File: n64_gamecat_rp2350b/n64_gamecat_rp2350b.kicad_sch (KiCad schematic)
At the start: 3 parts, among them U4 RP235x-B

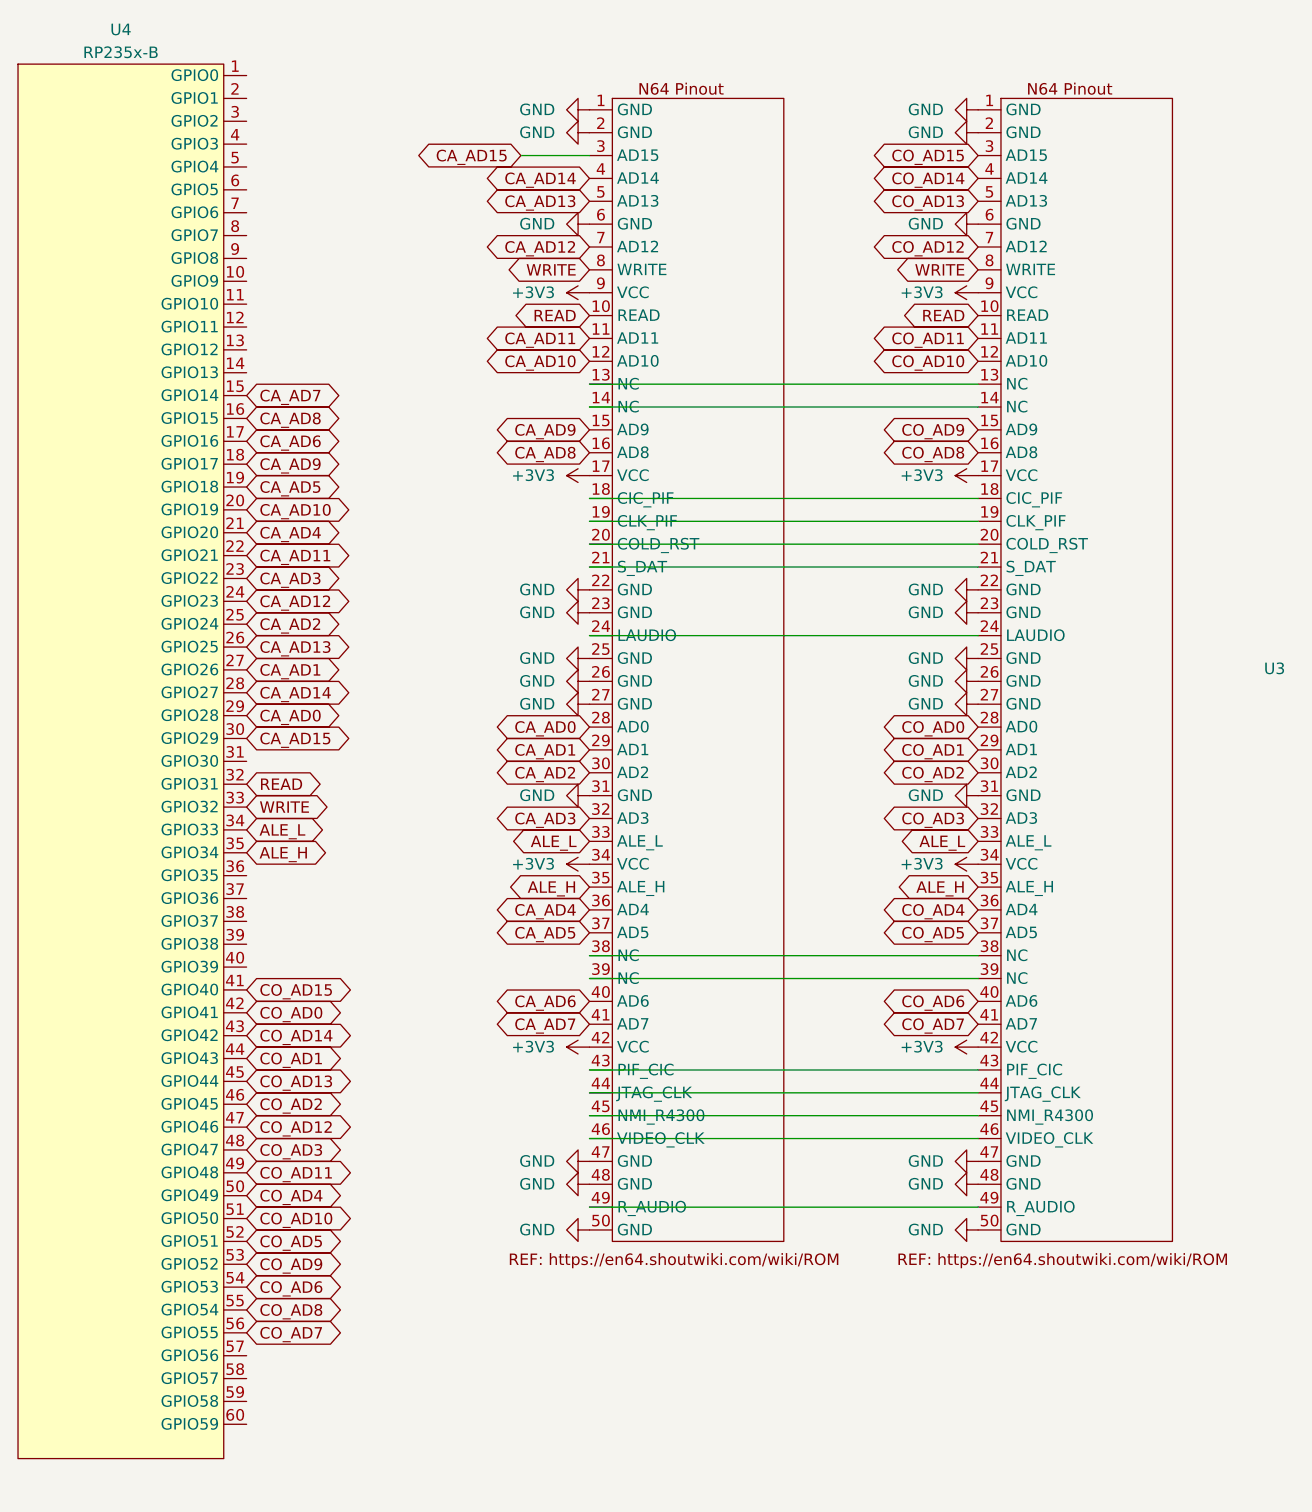
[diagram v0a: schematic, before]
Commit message: V0.6 PCB
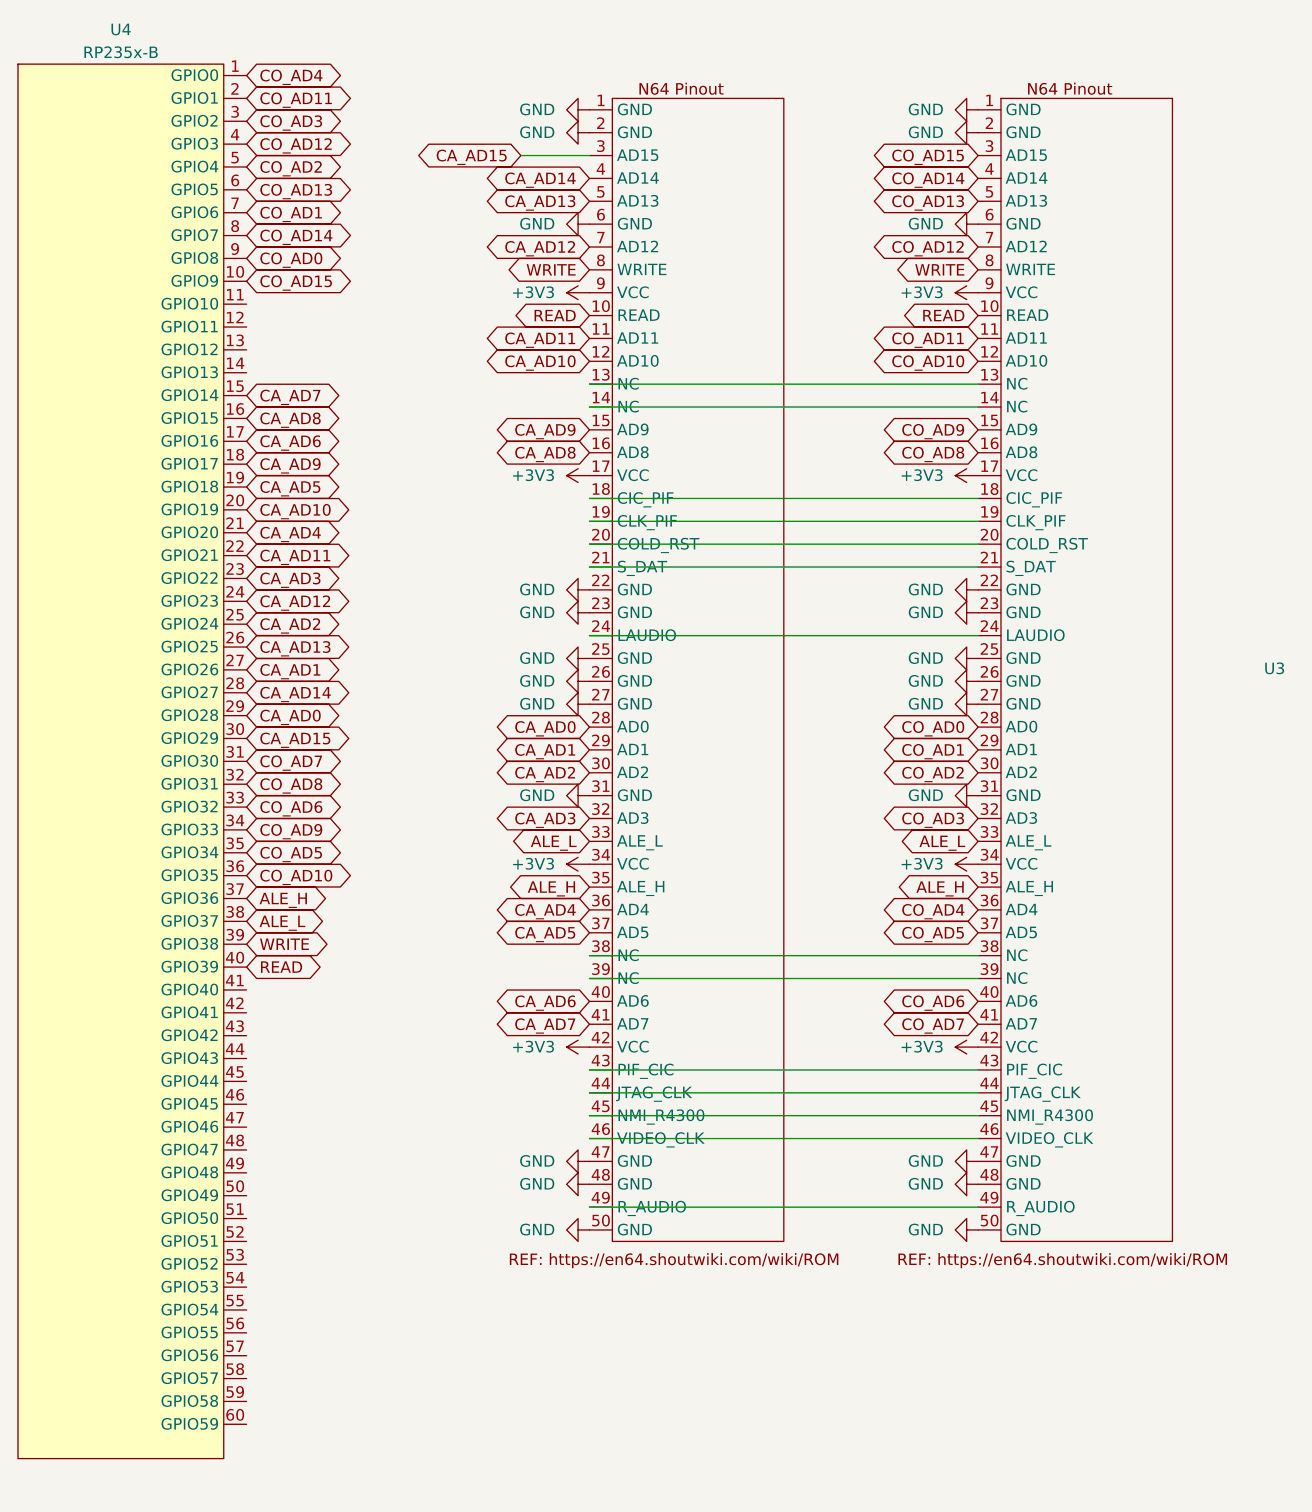
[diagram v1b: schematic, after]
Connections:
- net ALE_H: now also U4.37 (GPIO36); no longer U4.35 (GPIO34)
- net ALE_L: now also U4.38 (GPIO37); no longer U4.34 (GPIO33)
- net CO_AD0: now also U4.9 (GPIO8); no longer U4.42 (GPIO41)
- net CO_AD1: now also U4.7 (GPIO6); no longer U4.44 (GPIO43)
- net CO_AD10: now also U4.36 (GPIO35); no longer U4.51 (GPIO50)
- net CO_AD11: now also U4.2 (GPIO1); no longer U4.49 (GPIO48)
- net CO_AD12: now also U4.4 (GPIO3); no longer U4.47 (GPIO46)
- net CO_AD13: now also U4.6 (GPIO5); no longer U4.45 (GPIO44)
- net CO_AD14: now also U4.8 (GPIO7); no longer U4.43 (GPIO42)
- net CO_AD15: now also U4.10 (GPIO9); no longer U4.41 (GPIO40)
- net CO_AD2: now also U4.5 (GPIO4); no longer U4.46 (GPIO45)
- net CO_AD3: now also U4.3 (GPIO2); no longer U4.48 (GPIO47)
- net CO_AD4: now also U4.1 (GPIO0); no longer U4.50 (GPIO49)
- net CO_AD5: now also U4.35 (GPIO34); no longer U4.52 (GPIO51)
- net CO_AD6: now also U4.33 (GPIO32); no longer U4.54 (GPIO53)
- net CO_AD7: now also U4.31 (GPIO30); no longer U4.56 (GPIO55)
- net CO_AD8: now also U4.32 (GPIO31); no longer U4.55 (GPIO54)
- net CO_AD9: now also U4.34 (GPIO33); no longer U4.53 (GPIO52)
- net READ: now also U4.40 (GPIO39); no longer U4.32 (GPIO31)
- net WRITE: now also U4.39 (GPIO38); no longer U4.33 (GPIO32)

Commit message: v0.7 PCB; prep for 2350
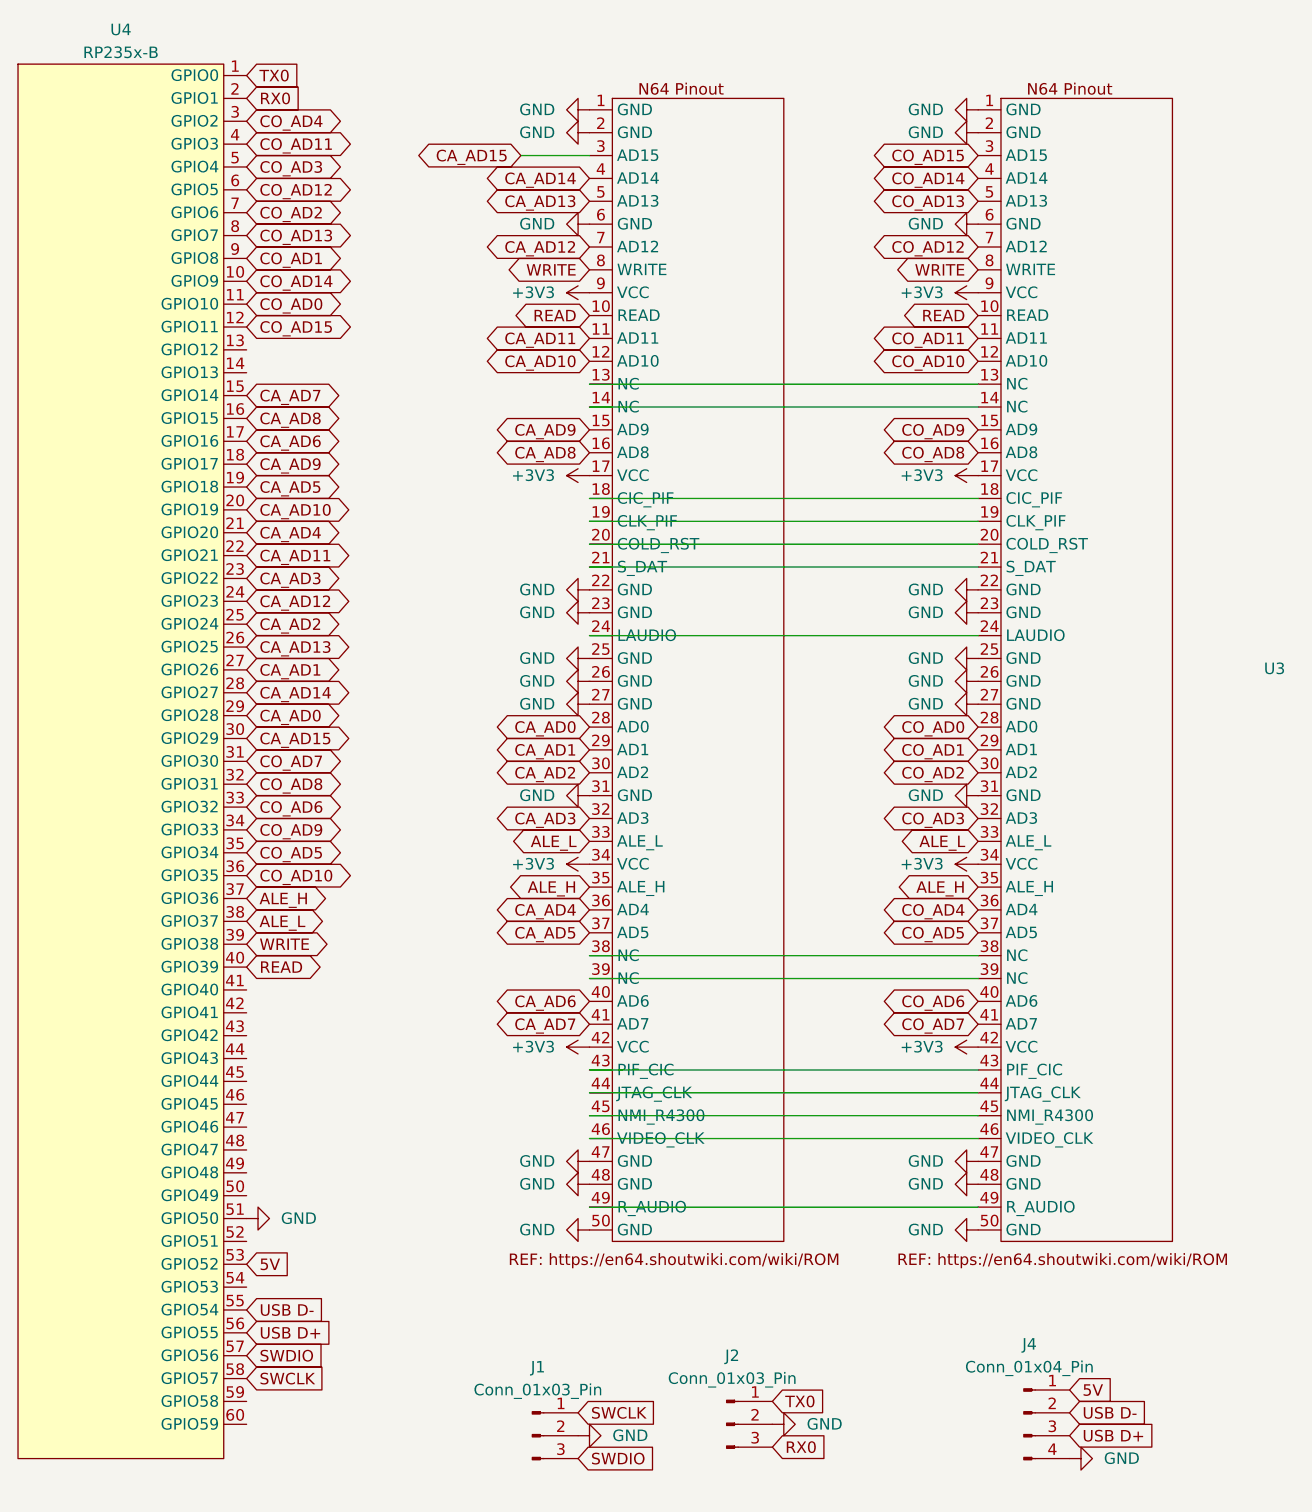
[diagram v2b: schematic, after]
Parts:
- added J1, J2: Conn_01x03_Pin, Connector_PinHeader_2.54mm:PinHeader_1x03_P2.54mm_Vertical, symbol Connector:Conn_01x03_Pin
- added J4: Conn_01x04_Pin, Connector_PinSocket_2.54mm:PinSocket_1x04_P2.54mm_Vertical, symbol Connector:Conn_01x04_Pin
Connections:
- net CO_AD0: now also U4.11 (GPIO10); no longer U4.9 (GPIO8)
- net CO_AD1: now also U4.9 (GPIO8); no longer U4.7 (GPIO6)
- net CO_AD11: now also U4.4 (GPIO3); no longer U4.2 (GPIO1)
- net CO_AD12: now also U4.6 (GPIO5); no longer U4.4 (GPIO3)
- net CO_AD13: now also U4.8 (GPIO7); no longer U4.6 (GPIO5)
- net CO_AD14: now also U4.10 (GPIO9); no longer U4.8 (GPIO7)
- net CO_AD15: now also U4.12 (GPIO11); no longer U4.10 (GPIO9)
- net CO_AD2: now also U4.7 (GPIO6); no longer U4.5 (GPIO4)
- net CO_AD3: now also U4.5 (GPIO4); no longer U4.3 (GPIO2)
- net CO_AD4: now also U4.3 (GPIO2); no longer U4.1 (GPIO0)
- net GND: now also U4.51 (GPIO50), J1.2 (Pin_2), J2.2 (Pin_2), J4.4 (Pin_4)
- net 5V: now reaches U4.53 (GPIO52)
- net 5V: now also J4.1 (Pin_1)
- net USB D-: now reaches U4.55 (GPIO54)
- net USB D-: now also J4.2 (Pin_2)
- net USB D+: now reaches U4.56 (GPIO55)
- net USB D+: now also J4.3 (Pin_3)
- net SWDIO: now reaches U4.57 (GPIO56)
- net SWDIO: now also J1.3 (Pin_3)
- net SWCLK: now reaches U4.58 (GPIO57)
- net SWCLK: now also J1.1 (Pin_1)
- new net RX0: J2.3 (Pin_3), U4.2 (GPIO1)
- new net TX0: J2.1 (Pin_1), U4.1 (GPIO0)

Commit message: Add v0.8 PCB
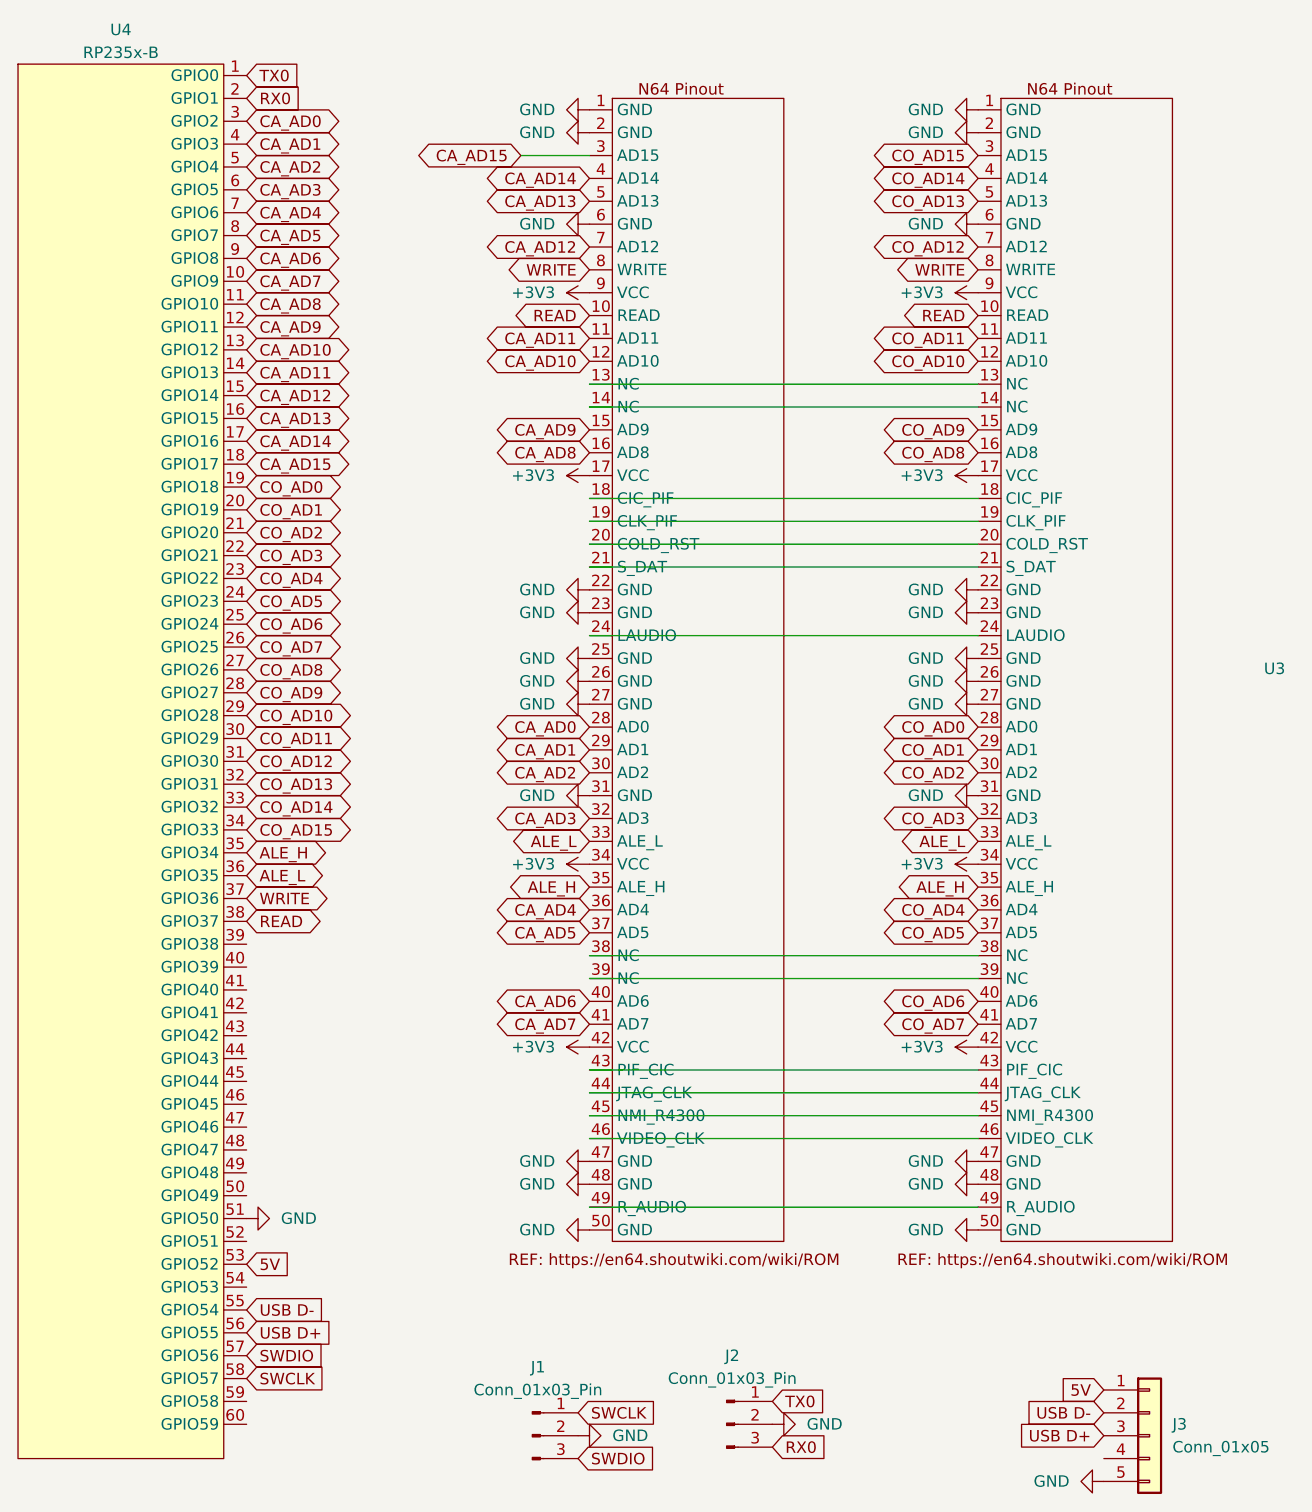
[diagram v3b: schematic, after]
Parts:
- removed J4: Conn_01x04_Pin, Connector_PinSocket_2.54mm:PinSocket_1x04_P2.54mm_Vertical, symbol Connector:Conn_01x04_Pin
- added J3: Conn_01x05, Connector_PinSocket_2.54mm:PinSocket_1x05_P2.54mm_Vertical, symbol Connector_Generic:Conn_01x05
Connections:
- net 5V: now also J3.1 (Pin_1)
- net ALE_H: now also U4.35 (GPIO34); no longer U4.37 (GPIO36)
- net ALE_L: now also U4.36 (GPIO35); no longer U4.38 (GPIO37)
- net CA_AD0: now also U4.3 (GPIO2); no longer U4.29 (GPIO28)
- net CA_AD1: now also U4.4 (GPIO3); no longer U4.27 (GPIO26)
- net CA_AD10: now also U4.13 (GPIO12); no longer U4.20 (GPIO19)
- net CA_AD11: now also U4.14 (GPIO13); no longer U4.22 (GPIO21)
- net CA_AD12: now also U4.15 (GPIO14); no longer U4.24 (GPIO23)
- net CA_AD13: now also U4.16 (GPIO15); no longer U4.26 (GPIO25)
- net CA_AD14: now also U4.17 (GPIO16); no longer U4.28 (GPIO27)
- net CA_AD15: now also U4.18 (GPIO17); no longer U4.30 (GPIO29)
- net CA_AD2: now also U4.5 (GPIO4); no longer U4.25 (GPIO24)
- net CA_AD3: now also U4.6 (GPIO5); no longer U4.23 (GPIO22)
- net CA_AD4: now also U4.7 (GPIO6); no longer U4.21 (GPIO20)
- net CA_AD5: now also U4.8 (GPIO7); no longer U4.19 (GPIO18)
- net CA_AD6: now also U4.9 (GPIO8); no longer U4.17 (GPIO16)
- net CA_AD7: now also U4.10 (GPIO9); no longer U4.15 (GPIO14)
- net CA_AD8: now also U4.11 (GPIO10); no longer U4.16 (GPIO15)
- net CA_AD9: now also U4.12 (GPIO11); no longer U4.18 (GPIO17)
- net CO_AD0: now also U4.19 (GPIO18); no longer U4.11 (GPIO10)
- net CO_AD1: now also U4.20 (GPIO19); no longer U4.9 (GPIO8)
- net CO_AD10: now also U4.29 (GPIO28); no longer U4.36 (GPIO35)
- net CO_AD11: now also U4.30 (GPIO29); no longer U4.4 (GPIO3)
- net CO_AD12: now also U4.31 (GPIO30); no longer U4.6 (GPIO5)
- net CO_AD13: now also U4.32 (GPIO31); no longer U4.8 (GPIO7)
- net CO_AD14: now also U4.33 (GPIO32); no longer U4.10 (GPIO9)
- net CO_AD15: now also U4.34 (GPIO33); no longer U4.12 (GPIO11)
- net CO_AD2: now also U4.21 (GPIO20); no longer U4.7 (GPIO6)
- net CO_AD3: now also U4.22 (GPIO21); no longer U4.5 (GPIO4)
- net CO_AD4: now also U4.23 (GPIO22); no longer U4.3 (GPIO2)
- net CO_AD5: now also U4.24 (GPIO23); no longer U4.35 (GPIO34)
- net CO_AD6: now also U4.25 (GPIO24); no longer U4.33 (GPIO32)
- net CO_AD7: now also U4.26 (GPIO25); no longer U4.31 (GPIO30)
- net CO_AD8: now also U4.27 (GPIO26); no longer U4.32 (GPIO31)
- net CO_AD9: now also U4.28 (GPIO27); no longer U4.34 (GPIO33)
- net GND: now also J3.5 (Pin_5)
- net READ: now also U4.38 (GPIO37); no longer U4.40 (GPIO39)
- net USB D+: now also J3.3 (Pin_3)
- net USB D-: now also J3.2 (Pin_2)
- net WRITE: now also U4.37 (GPIO36); no longer U4.39 (GPIO38)
